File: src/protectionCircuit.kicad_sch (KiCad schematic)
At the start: 22 parts, among them M1 CSD19534Q5A, M2 CSD19534Q5A, U1 LM74910QRGERQ1

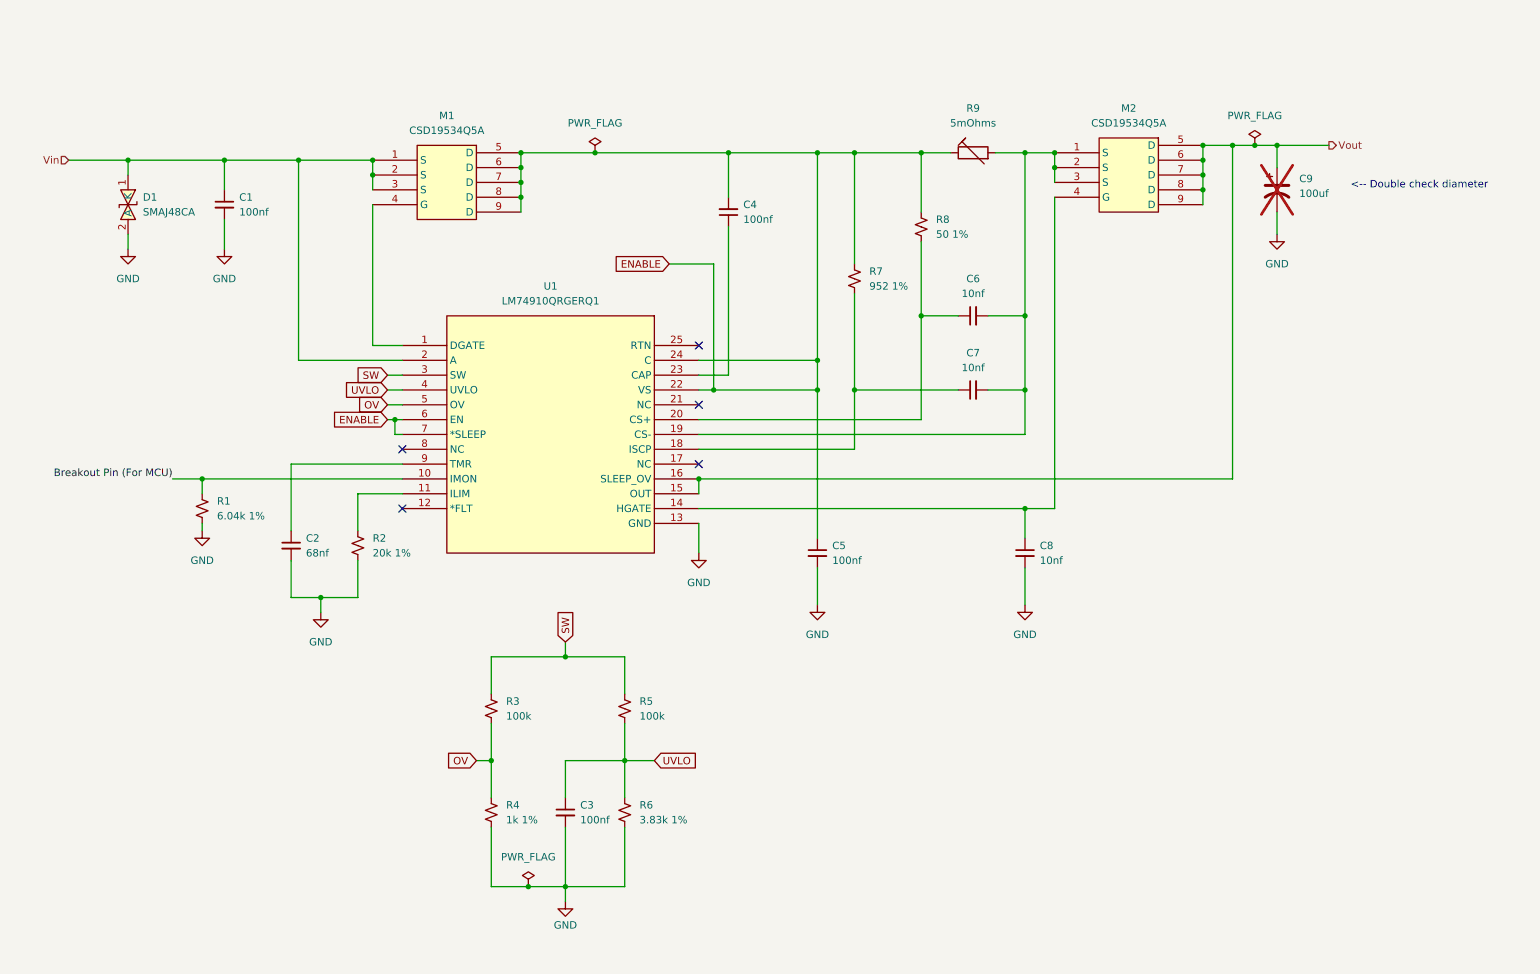
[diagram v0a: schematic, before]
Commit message: GG
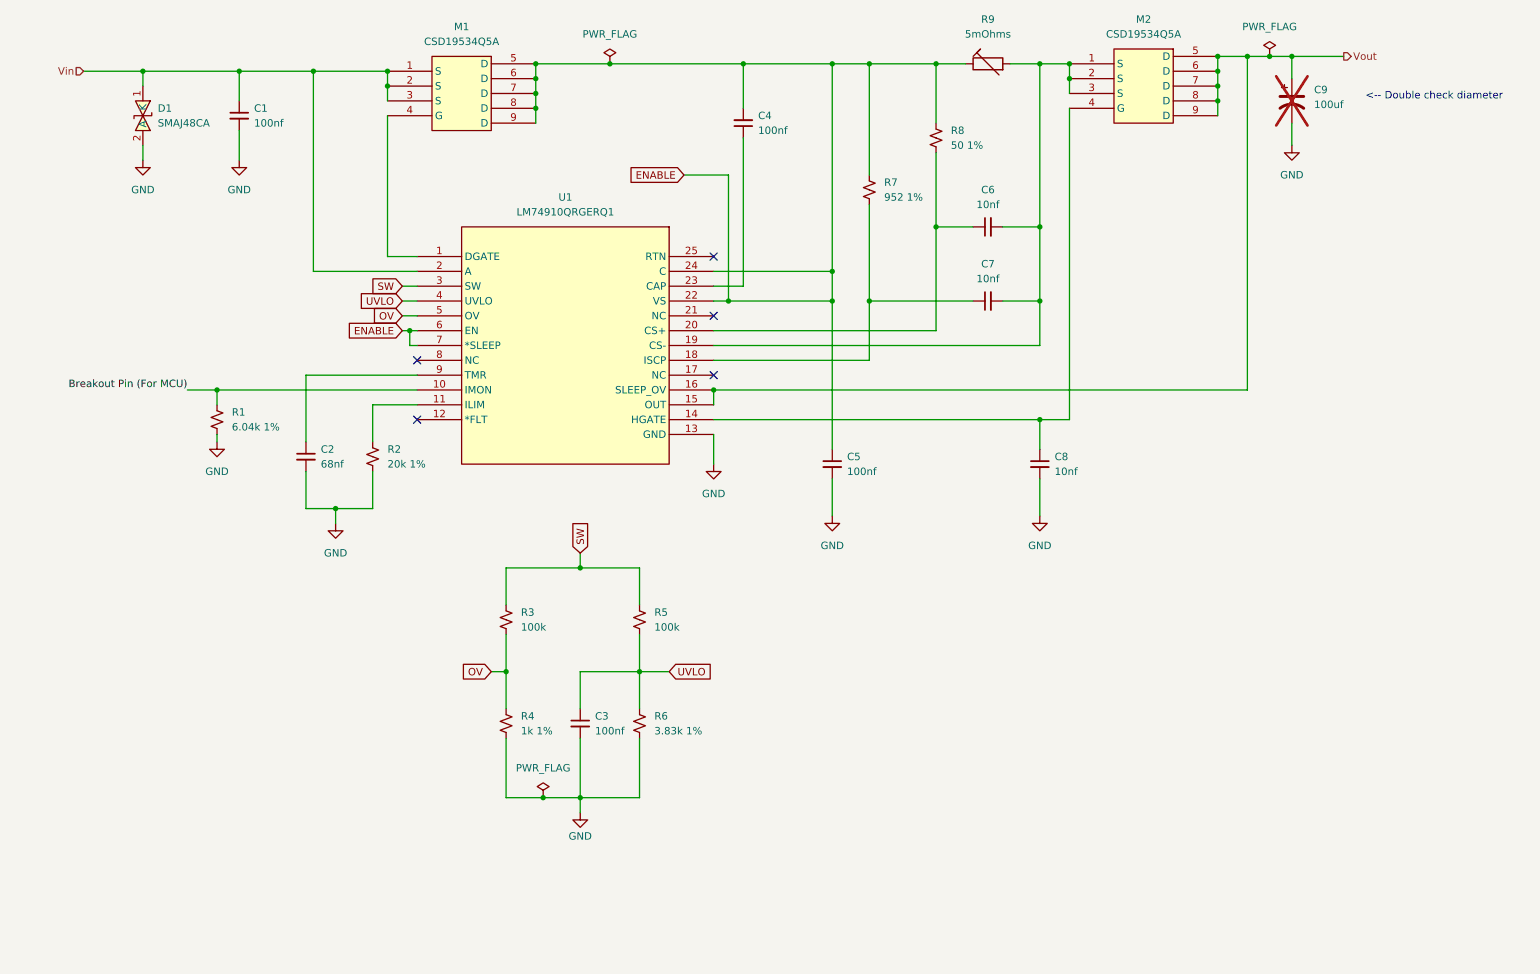
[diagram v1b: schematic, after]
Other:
- moved on the sheet: C1, C2, C3, C4, C5, C6, C7, C8, C9, D1, M1, M2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

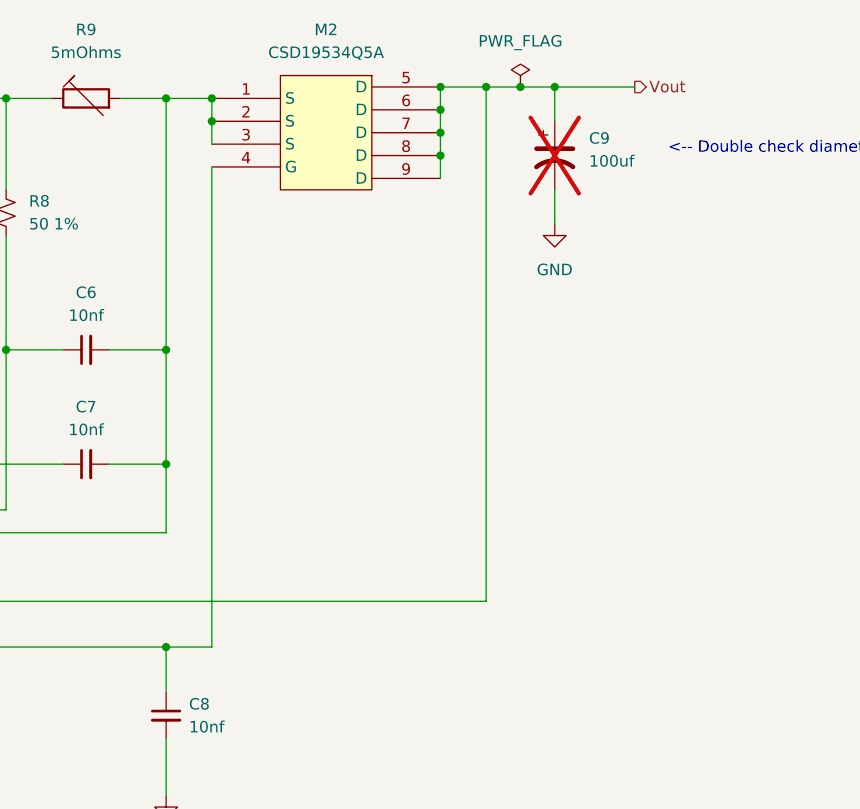
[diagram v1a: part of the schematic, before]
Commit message: Working on PCB layout
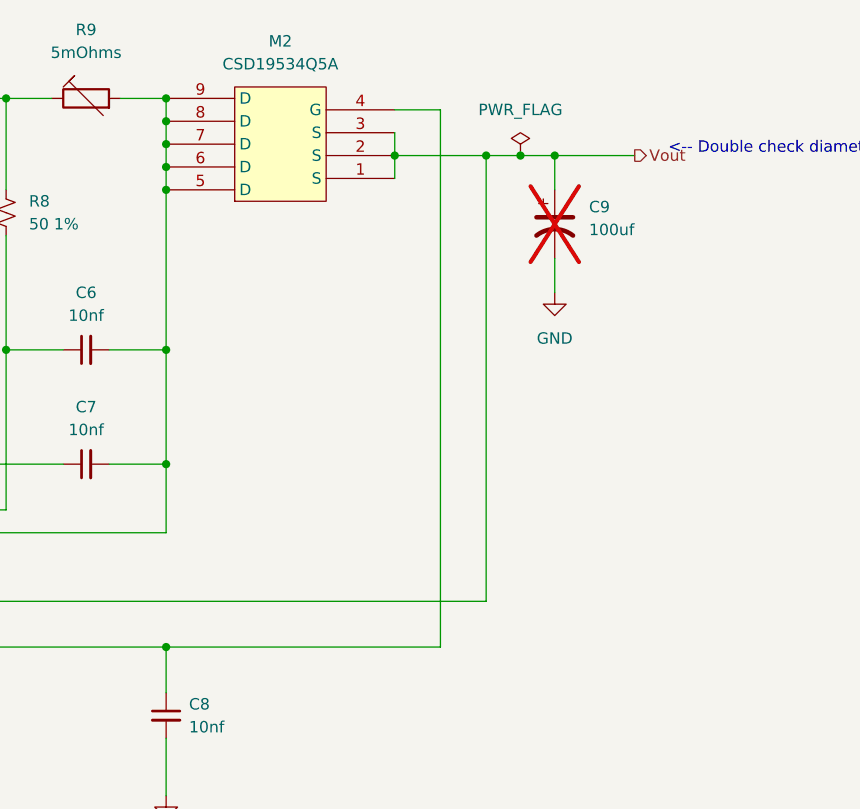
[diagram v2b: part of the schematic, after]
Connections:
- net Vout: now also M2.1 (S), M2.2 (S), M2.3 (S); no longer M2.5 (D), M2.6 (D), M2.7 (D), M2.8 (D), M2.9 (D)
- net at C6.2, C7.2, R9.2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: now also M2.5 (D), M2.6 (D), M2.7 (D), M2.8 (D), M2.9 (D); no longer M2.1 (S), M2.2 (S), M2.3 (S)
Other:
- moved on the sheet: C9, M2

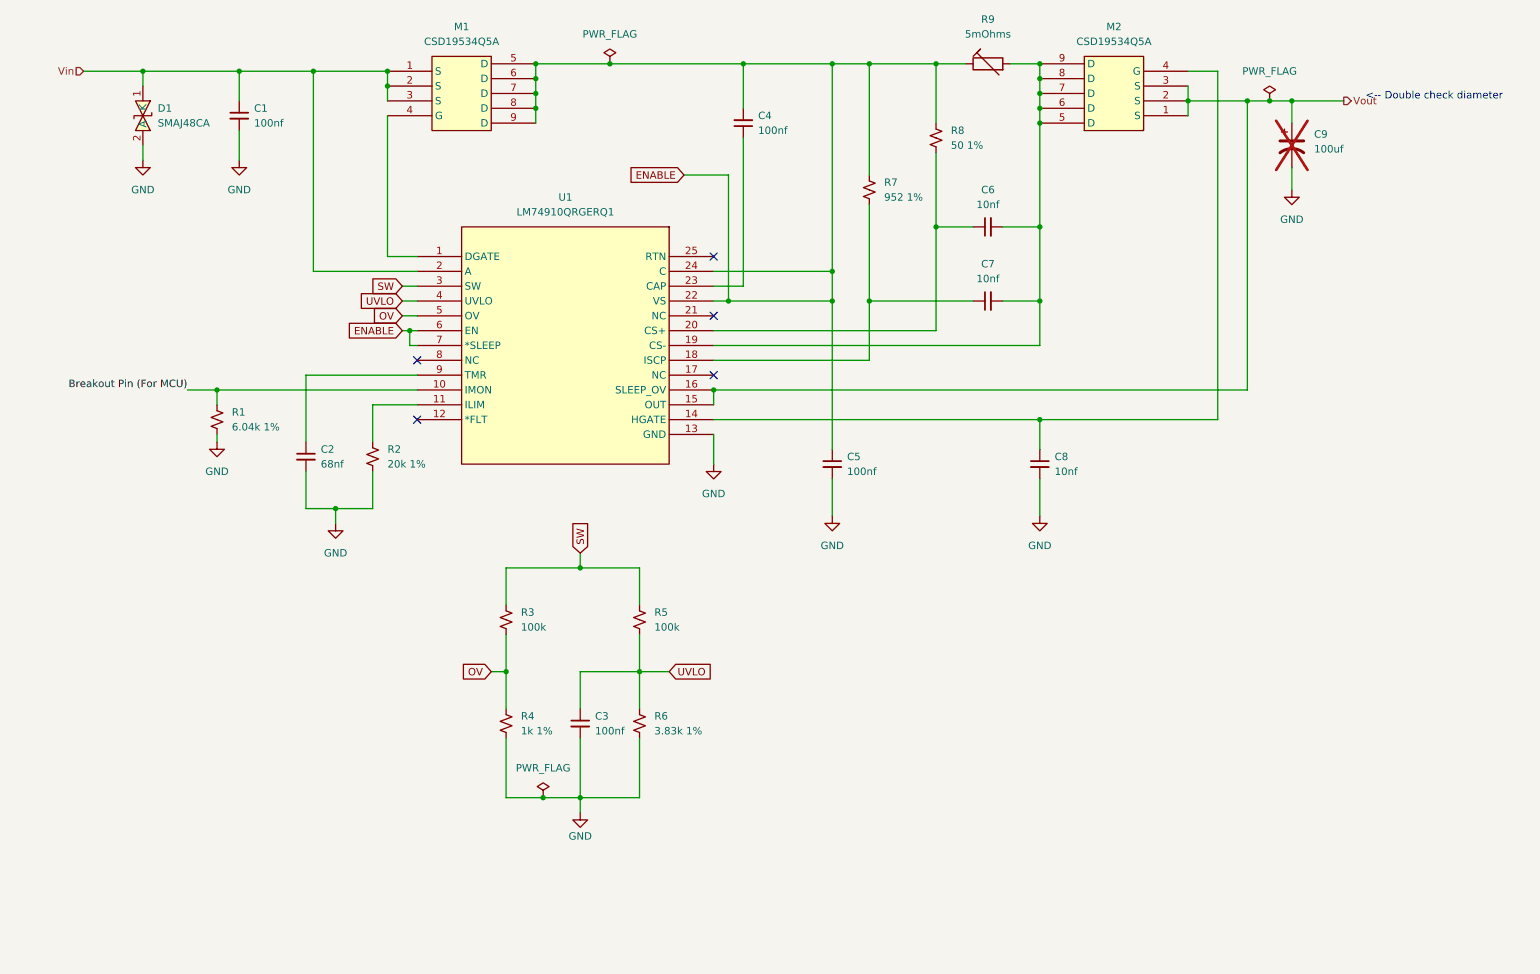
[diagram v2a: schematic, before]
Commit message: Completed half of the PCB layout
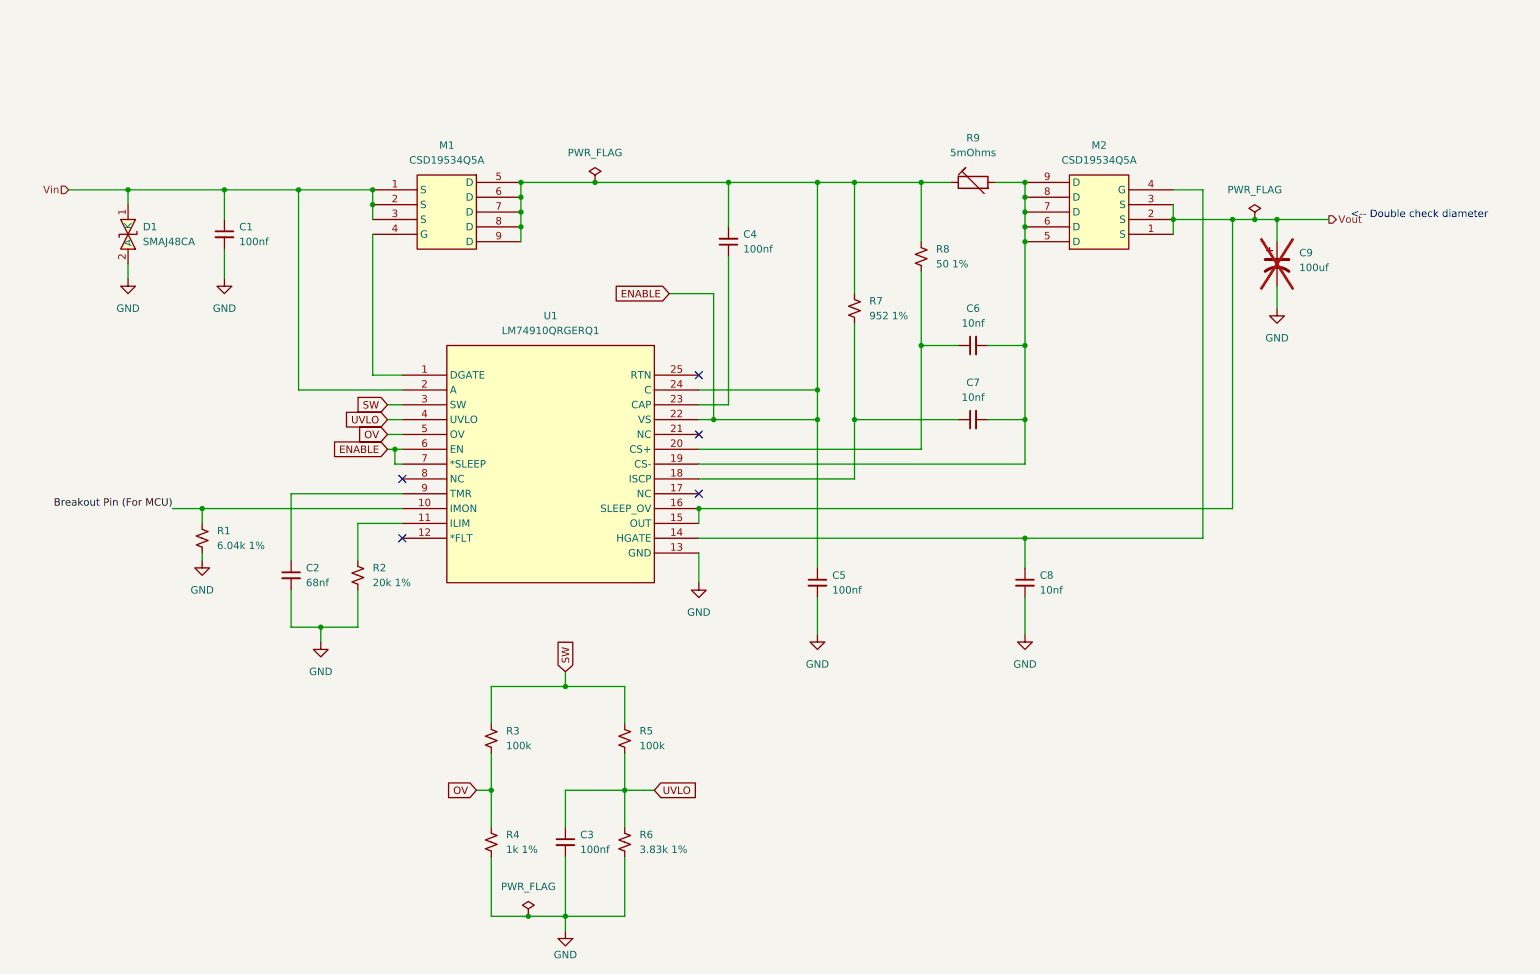
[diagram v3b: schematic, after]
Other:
- moved on the sheet: C1, C2, C3, C4, C5, C6, C7, C8, C9, D1, M1, M2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

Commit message: Upated parts and BOM
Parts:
- C1: LCSC Part (none) -> C527375; MPN (none) -> CC1210KKX7R0BB104; Manufacturer (none) -> YAGEO
- C2: LCSC Part (none) -> C309475; MPN (none) -> CC0603JRX7R9BB683; Manufacturer (none) -> YAGEO
- C3, C4, C5: LCSC Part (none) -> C108079; MPN (none) -> CC0603KRX7R7BB104; Manufacturer (none) -> YAGEO
- C6, C7, C8: LCSC Part (none) -> C1853238; MPN (none) -> AC0603JRX7R0BB103; Manufacturer (none) -> YAGEO
- R1: LCSC Part (none) -> C25977; MPN (none) -> 0603WAF6041T5E; Manufacturer (none) -> UNI-ROYAL(Uniroyal Elec)
- R2: LCSC Part (none) -> C403057; MPN (none) -> ERJ3EKF2002V; Manufacturer (none) -> PANASONIC
- R3, R5: LCSC Part (none) -> C844916; MPN (none) -> CRCW0603100KFKEA; Manufacturer (none) -> Vishay Intertech
- R4: LCSC Part (none) -> C2653986; MPN (none) -> ESR03EZPF1001; Manufacturer (none) -> ROHM Semicon
- R6: LCSC Part (none) -> C49654961; MPN (none) -> GR0603F3K83T5G00; Manufacturer (none) -> GiantOhm
- R8: LCSC Part (none) -> C844932; MPN (none) -> CRCW060350R0FKEA; Manufacturer (none) -> Vishay Intertech
- R9: LCSC Part (none) -> C6490398; MPN (none) -> CSNL2010FT5L00; Manufacturer (none) -> SEI(Stackpole Elec)
- U1: LCSC Part (none) -> C22427891; MPN (none) -> LM74910QRGERQ1; Manufacturer (none) -> Texas Instruments

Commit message: Finalized and exported BOM to project
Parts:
- M1, M2: LCSC Part (none) -> C2876530; MPN (none) -> CSD19534Q5AT; Manufacturer (none) -> Texas Instruments
- R7: LCSC Part (none) -> C334839; MPN (none) -> WR06X9530FTL; Manufacturer (none) -> Walsin Tech Corp
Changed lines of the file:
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@@
+			)
+		)
+		(property "LCSC Part" "C2876530"
+			(at 72.39 53.34 0)
+			(hide yes)
+			(show_name no)
+			(do_not_autoplace no)
+			(effects
+				(font
+					(size 1.27 1.27)
+				)
+			)
+		)
+		(property "MPN" "CSD19534Q5AT"
+			(at 72.39 53.34 0)
+			(hide yes)
+			(show_name no)
+			(do_not_autoplace no)
+			(effects
+				(font
+					(size 1.27 1.27)
+				)
+			)
+		)
+		(property "Manufacturer" "Texas Instruments"
+			(at 72.39 53.34 0)
+			(hide yes)
+			(show_name no)
+			(do_not_autoplace no)
+			(effects
+				(font
+					(size 1.27 1.27)
+				)
 			)
 		)
@@
 			)
 		)
+		(property "LCSC Part" "C334839"
+			(at 154.94 76.2 0)
+			(hide yes)
+			(show_name no)
+			(do_not_autoplace no)
+			(effects
+				(font
+					(size 1.27 1.27)
+				)
+			)
+		)
+		(property "MPN" "WR06X9530FTL"
+			(at 154.94 76.2 0)
+			(hide yes)
+			(show_name no)
+			(do_not_autoplace no)
+			(effects
+				(font
+					(size 1.27 1.27)
+				)
+			)
+		)
+		(property "Manufacturer" "Walsin Tech Corp"
+			(at 154.94 76.2 0)
+			(hide yes)
+			(show_name no)
+			(do_not_autoplace no)
+			(effects
+				(font
+					(size 1.27 1.27)
+				)
+			)
+		)
 		(pin "1"
 		)
@@
 			)
 		)
+		(property "LCSC Part" "C2876530"
+			(at 209.55 66.04 0)
+			(hide yes)
+			(show_name no)
+			(do_not_autoplace no)
+			(effects
+				(font
+					(size 1.27 1.27)
+				)
+			)
+		)
+		(property "MPN" "CSD19534Q5AT"
+			(at 209.55 66.04 0)
+			(hide yes)
+			(show_name no)
+			(do_not_autoplace no)
+			(effects
+				(font
+					(size 1.27 1.27)
+				)
+			)
+		)
+		(property "Manufacturer" "Texas Instruments"
+			(at 209.55 66.04 0)
+			(hide yes)
+			(show_name no)
+			(do_not_autoplace no)
+			(effects
+				(font
+					(size 1.27 1.27)
+				)
+			)
+		)

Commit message: Updated BOM
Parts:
- C9: now left out of the parts list
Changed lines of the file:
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@@
 		(body_style 1)
 		(exclude_from_sim no)
-		(in_bom yes)
+		(in_bom no)
 		(on_board yes)
 		(in_pos_files yes)
